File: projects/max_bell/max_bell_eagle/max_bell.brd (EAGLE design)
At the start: 63.5 x 63.5 mm, 23 parts

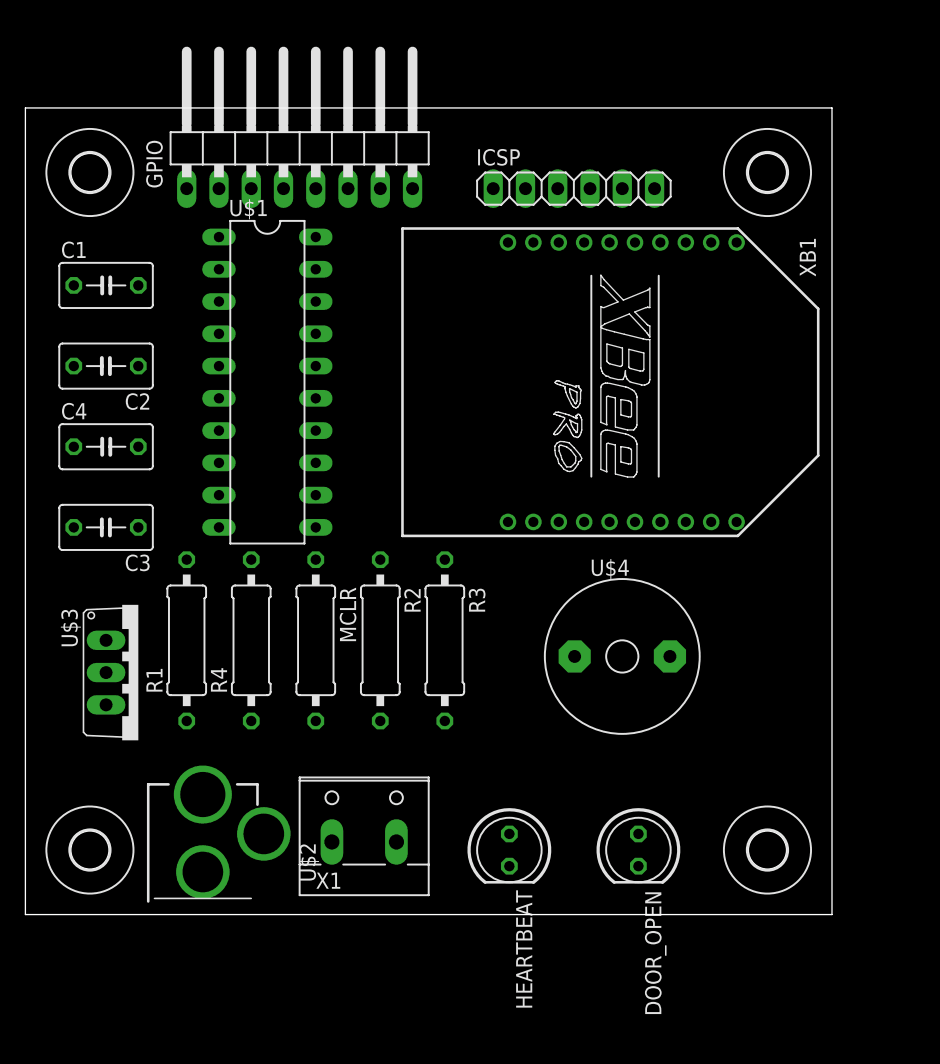
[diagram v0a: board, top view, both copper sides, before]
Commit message: updates to max_bell
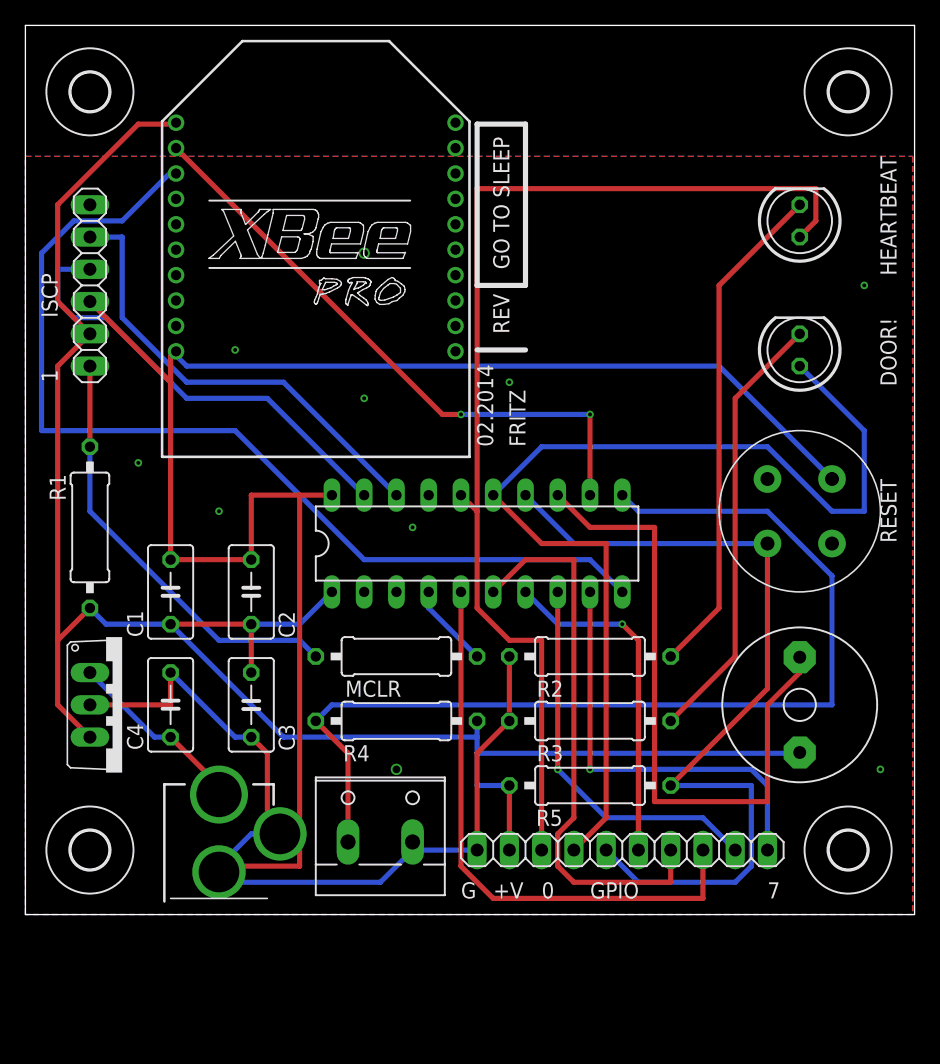
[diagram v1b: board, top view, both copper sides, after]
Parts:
- removed GPIO: (no value), pinhead:1X08/90
- added JP1: (no value), pinhead:1X10
- added R5: 10K, rcl:0309/12
- added U$9: (no value), holes:3,0
- R2: value 1K -> 10K
- U$5: value (none) -> SWITCH_MOMENTARY; device holes:3,0 -> fritz:MOMENTARY_SWITCH
- moved U$5 61.9 mm to (61.0, 31.8), turned to 90 degrees
- moved U$8 60.0 mm to (64.8, 64.8)
- moved HEARTBEAT 54.6 mm to (61.0, 54.6), turned to 90 degrees
- moved U$7 53.7 mm to (64.8, 5.08)
- moved U$6 53.3 mm to (5.08, 5.08)
- moved DOOR_OPEN 41.4 mm to (61.0, 44.5), turned to 90 degrees
- moved ICSP 38.9 mm to (5.08, 49.5), turned to 90 degrees
- moved XB1 26.7 mm to (22.9, 53.3), turned to 0 degrees
- moved C1 24.7 mm to (11.4, 25.4), turned to 90 degrees
- moved C2 21.1 mm to (17.8, 25.4), turned to 90 degrees
- moved C4 20.9 mm to (11.4, 16.5), turned to 90 degrees
- moved U$1 20.8 mm to (35.6, 29.2), turned to 0 degrees
- moved C3 18.1 mm to (17.8, 16.5), turned to 270 degrees
- moved R2 16.6 mm to (44.5, 20.3), turned to 0 degrees
- moved U$4 14.5 mm to (61.0, 16.5), turned to 270 degrees
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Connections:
- net GND: now also JP1.1, U$5.4; no longer U$4.2
- net GPIO_0: now also JP1.3; no longer GPIO.1
- net GPIO_1: now also JP1.4; no longer GPIO.2
- net GPIO_2: now also JP1.5, R5.1, U$5.1; no longer GPIO.3
- net GPIO_3: now also JP1.6; no longer GPIO.4
- net GPIO_4: now also JP1.7; no longer GPIO.5
- net GPIO_5: now also JP1.8; no longer GPIO.6
- net GPIO_6: now also JP1.9; no longer GPIO.7
- net GPIO_7: now also JP1.10; no longer GPIO.8
- net ICSPCLK: now also U$1.18
- net ICSPDAT: now also U$1.19
- net VDD: now also JP1.2, R5.2, U$4.2
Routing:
- net GND: track 0.00 -> 208.4 mm, vias 0 -> 10
- net VDD: track 0.00 -> 151.0 mm
- net GPIO_0: track 0.00 -> 88.5 mm
- net GPIO_1: track 0.00 -> 82.1 mm
- net TERMINAL_BLOCK: track 0.00 -> 81.0 mm
- net TX: track 0.00 -> 78.2 mm
- net GPIO_2: track 0.00 -> 68.5 mm
- net BUZZER: track 0.00 -> 51.6 mm
- net RX: track 0.00 -> 47.6 mm, vias 0 -> 2
- net GPIO_5: track 0.00 -> 45.5 mm
- net GPIO_4: track 0.00 -> 44.0 mm
- net N$4: track 0.00 -> 39.8 mm
- net ICSPCLK: track 0.00 -> 36.3 mm
- net ICSPDAT: track 0.00 -> 35.5 mm
- net N$5: track 0.00 -> 34.7 mm
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- added copper zone on layer 1, net GND
- added copper zone on layer 16, net GND
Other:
- board size 63.5 x 63.5 mm -> 70 x 70 mm
- board text added: "+V"
- board text added: "0"
- board text added: "02.2014"
- board text added: "1"
- board text added: "7"
- board text added: "DOOR!"
- board text added: "FRITZ"
- board text added: "G"
- board text added: "GO TO SLEEP"
- board text added: "GPIO"
- board text added: "HEARTBEAT"
- board text added: "ISCP"
- board text added: "RESET"
- board text added: "REV"
